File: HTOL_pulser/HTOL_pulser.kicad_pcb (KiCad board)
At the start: 2 copper layers, 63 x 49.5 mm, 25 parts, among them IC1 4093D, J1 IN_ON, J10 OUT_OFF, J11 OUT_ON, J12 IN_ON, J2 OUT_ON, J3 OUT_OFF, J4 IN_OFF, J5 GND, J6 +5V, J7 +5V, J8 GND, J9 IN_OFF, U1 74AHCT123

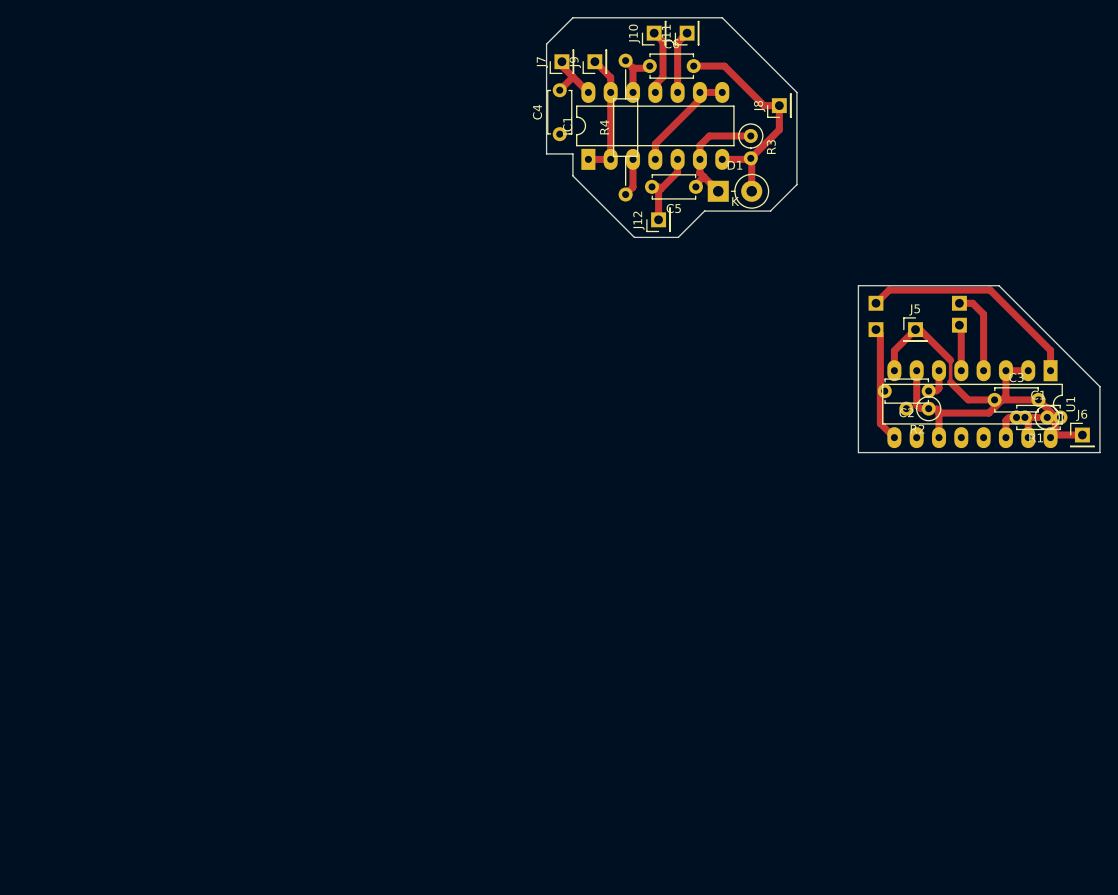
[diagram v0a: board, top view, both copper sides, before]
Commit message: a
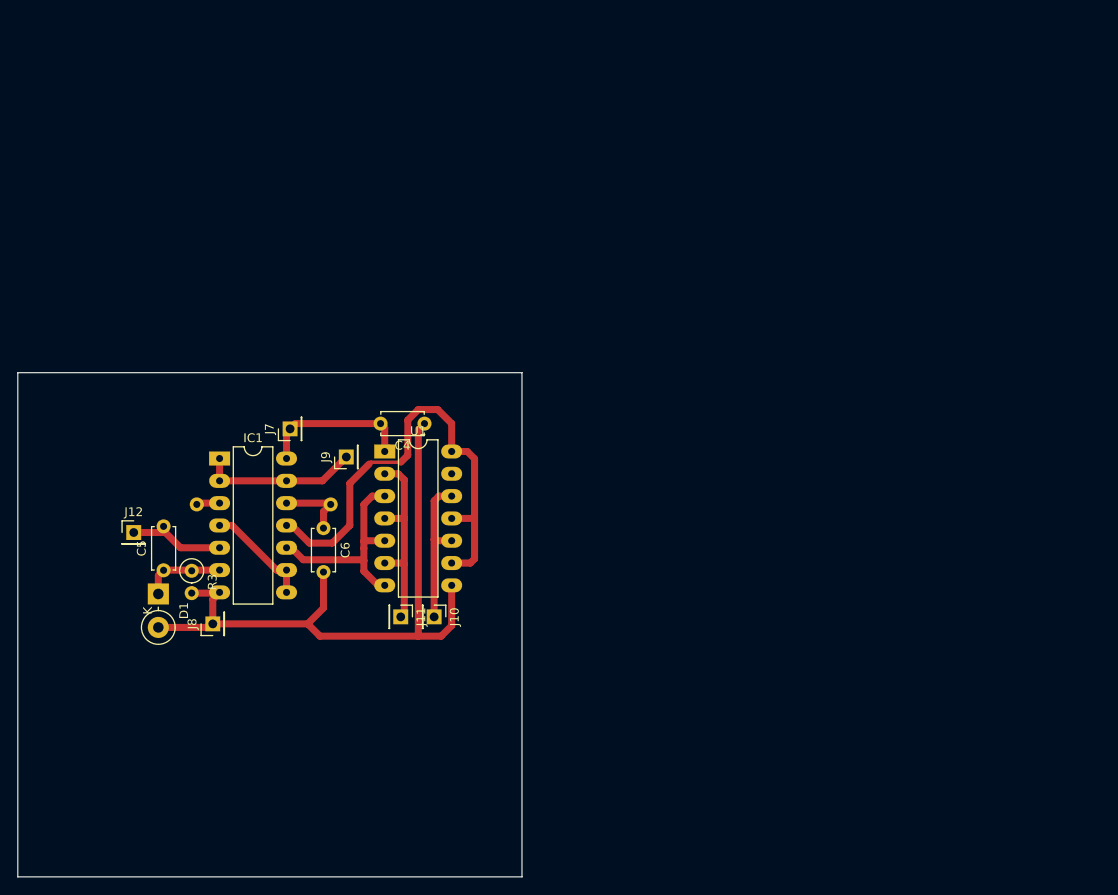
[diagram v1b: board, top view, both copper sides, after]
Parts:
- removed C1, C2: 68p, Capacitor_THT:C_Disc_D4.7mm_W2.5mm_P5.00mm
- removed C3: 100n, Capacitor_THT:C_Disc_D4.7mm_W2.5mm_P5.00mm
- removed J1: IN_ON, Connector_PinHeader_2.54mm:PinHeader_1x01_P2.54mm_Vertical
- removed J2: OUT_ON, Connector_PinHeader_2.54mm:PinHeader_1x01_P2.54mm_Vertical
- removed J3: OUT_OFF, Connector_PinHeader_2.54mm:PinHeader_1x01_P2.54mm_Vertical
- removed J4: IN_OFF, Connector_PinHeader_2.54mm:PinHeader_1x01_P2.54mm_Vertical
- removed J5: GND, Connector_PinHeader_2.54mm:PinHeader_1x01_P2.54mm_Vertical
- removed J6: +5V, Connector_PinHeader_2.54mm:PinHeader_1x01_P2.54mm_Vertical
- removed R1, R2: 10k, Resistor_THT:R_Axial_DIN0207_L6.3mm_D2.5mm_P2.54mm_Vertical
- R4: moved to B.Cu
- U1: value 74AHCT123 -> 4050; footprint Package_DIP:DIP-16_W7.62mm_LongPads -> Package_DIP:DIP-14_W7.62mm_LongPads
- moved J8 87.4 mm to (100.0, 154.0)
- moved R3 80.6 mm to (97.6, 148.0)
- moved D1 78.5 mm to (93.8, 150.6), turned to -90 degrees
- moved U1 76.4 mm to (119.6, 134.4), turned to 0 degrees
- moved C5 74.7 mm to (94.4, 147.9), turned to 90 degrees
- moved J11 74.0 mm to (121.4, 153.2), turned to -90 degrees
- moved J10 71.0 mm to (125.2, 153.2), turned to -90 degrees
- moved J12 69.6 mm to (91.0, 143.6), turned to 0 degrees
- moved C6 64.4 mm to (112.6, 143.1), turned to -90 degrees
- moved R4 60.2 mm to (98.2, 140.4), turned to 0 degrees
- moved IC1 54.1 mm to (100.8, 135.2), turned to 0 degrees
- moved J9 53.2 mm to (115.2, 135.0)
- moved J7 52.0 mm to (108.8, 131.8)
- moved C4 36.4 mm to (124.1, 131.2), turned to 180 degrees
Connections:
- J10 pad 1: Net-(IC1D-O) -> Net-(J10-Pin_1)
- J11 pad 1: Net-(IC1C-O) -> Net-(J11-Pin_1)
- U1 pad 1: Net-(J4-Pin_1) -> +5V
- U1 pad 10: +5V -> Net-(J10-Pin_1)
- U1 pad 11: +5V -> Net-(IC1D-O)
- U1 pad 12: unconnected-(U1B-~{Q}-Pad12) -> Net-(J10-Pin_1)
- U1 pad 13: unconnected-(U1A-Q-Pad13) -> (no net)
- U1 pad 14: Net-(U1A-Cext) -> Net-(IC1D-O)
- U1 pad 2: +5V -> Net-(J11-Pin_1)
- U1 pad 3: +5V -> Net-(IC1C-O)
- U1 pad 4: Net-(J3-Pin_1) -> Net-(J11-Pin_1)
- U1 pad 5: Net-(J2-Pin_1) -> Net-(IC1C-O)
- U1 pad 6: Net-(U1B-Cext) -> Net-(J11-Pin_1)
- U1 pad 7: Net-(U1B-RCext) -> Net-(IC1C-O)
- U1 pad 9: Net-(J1-Pin_1) -> Net-(IC1D-O)
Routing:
- net Net-(IC1D-O): track 7.52 -> 54.7 mm
- net GND: track 44.6 -> 77.5 mm
- net Net-(J4-Pin_1): track 25.6 -> 0.00 mm
- net Net-(J11-Pin_1): track 0.00 -> 22.8 mm
- net +5V: track 37.3 -> 18.9 mm
- net Net-(IC1C-O): track 7.20 -> 25.2 mm
- net Net-(J10-Pin_1): track 0.00 -> 17.5 mm
- net Net-(J1-Pin_1): track 13.2 -> 0.00 mm
- net Net-(J3-Pin_1): track 9.69 -> 0.00 mm
- net Net-(J2-Pin_1): track 5.26 -> 0.00 mm
- net Net-(U1B-RCext): track 4.51 -> 0.00 mm
- net Net-(D1-K): track 13.8 -> 9.33 mm
- net Net-(U1A-RCext): track 4.22 -> 0.00 mm
- net Net-(IC1A-I0): track 14.4 -> 18.1 mm
- net Net-(U1B-Cext): track 2.45 -> 0.00 mm
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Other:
- board size 63 x 49.5 mm -> 57.4 x 57.4 mm
